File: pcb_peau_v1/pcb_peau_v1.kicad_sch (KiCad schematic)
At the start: 26 parts, among them J1 Conn_01x05, J2 Conn_01x05, J4 Conn_02x08_Top_Bottom, J5 Conn_02x12_Top_Bottom, U2 TLC274, U3 CD74HC4067SM, U4 CD74HC4067SM, U5 CD74HC4067SM, U6 CD74HC4067SM, U7 TLC274, U8 TLC274, U9 TLC274

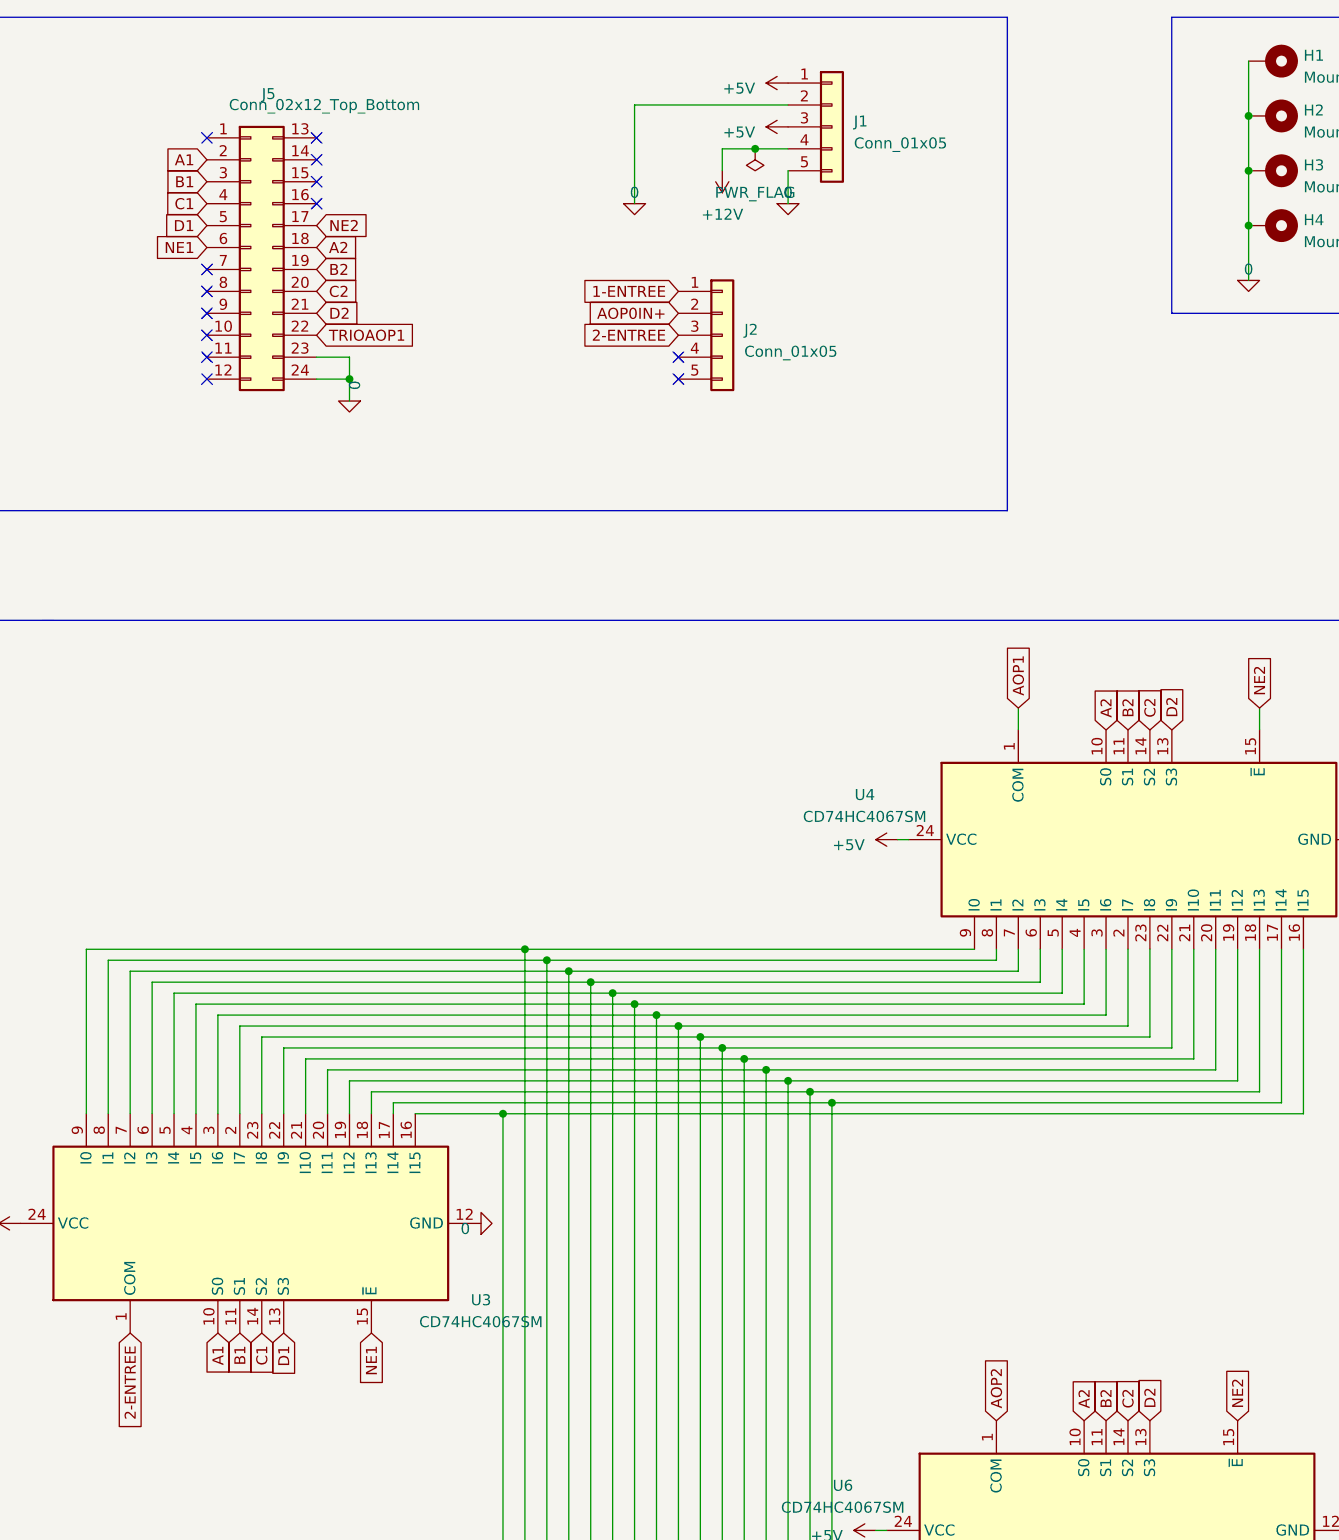
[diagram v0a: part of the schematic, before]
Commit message: PCB corrigé
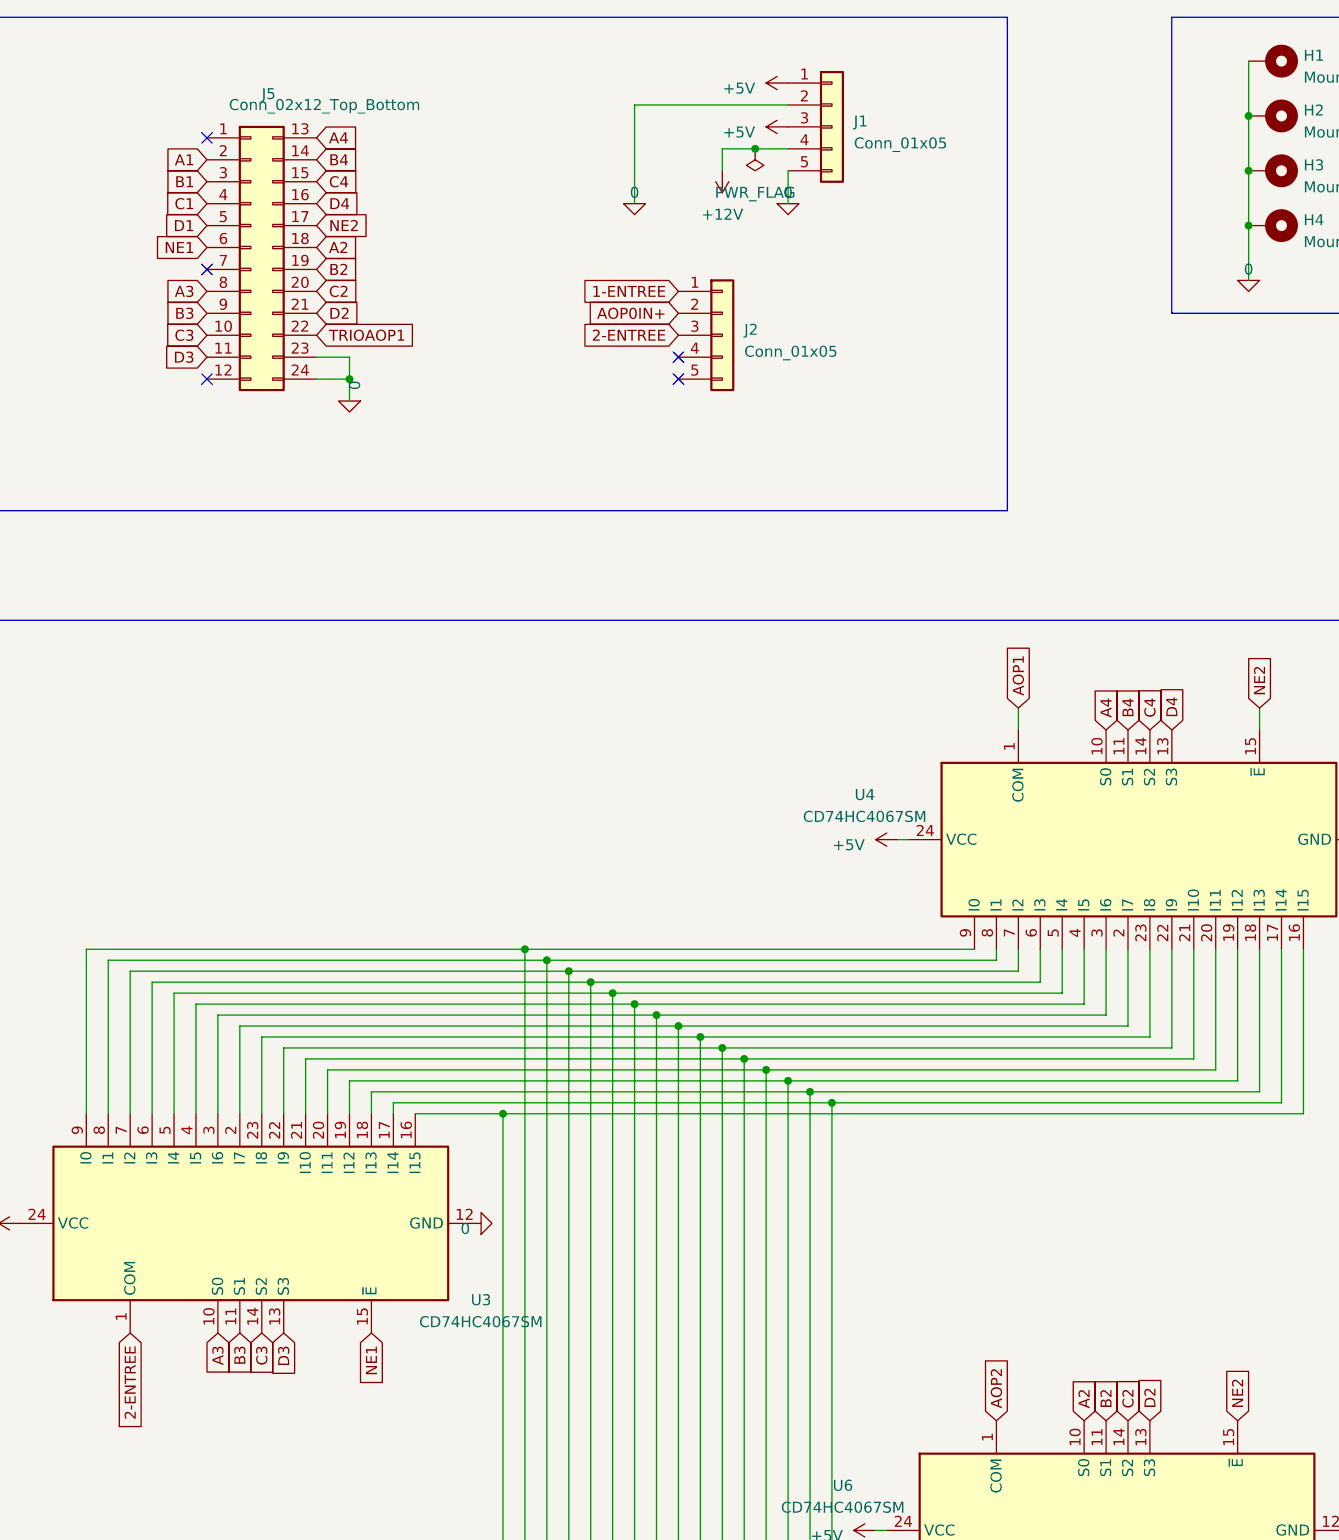
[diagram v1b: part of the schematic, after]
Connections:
- net A1: no longer U3.10 (S0)
- net A2: no longer U4.10 (S0)
- net B1: no longer U3.11 (S1)
- net B2: no longer U4.11 (S1)
- net C1: no longer U3.14 (S2)
- net C2: no longer U4.14 (S2)
- net D1: no longer U3.13 (S3)
- net D2: no longer U4.13 (S3)
- net C3: now reaches J5.10 (Pin_10)
- net C3: now also U3.14 (S2)
- net D3: now reaches J5.11 (Pin_11)
- net D3: now also U3.13 (S3)
- net A4: now reaches J5.13 (Pin_13)
- net A4: now also U4.10 (S0)
- net B4: now reaches J5.14 (Pin_14)
- net B4: now also U4.11 (S1)
- net C4: now reaches J5.15 (Pin_15)
- net C4: now also U4.14 (S2)
- net D4: now reaches J5.16 (Pin_16)
- net D4: now also U4.13 (S3)
- net A3: now reaches J5.8 (Pin_8)
- net A3: now also U3.10 (S0)
- net B3: now reaches J5.9 (Pin_9)
- net B3: now also U3.11 (S1)
- no-connect marks 13 -> 5
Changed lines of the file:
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@@
   (junction (at 96.52 214.63) (diameter 0) (color 0 0 0 0)
   )
-  (no_connect (at 64.77 40.64))
-  (no_connect (at 52.07 60.96))
   (no_connect (at 52.07 35.56))
   (no_connect (at 106.68 63.5))
-  (no_connect (at 52.07 53.34))
-  (no_connect (at 52.07 58.42))
   (no_connect (at 106.68 60.96))
-  (no_connect (at 52.07 55.88))
-  (no_connect (at 64.77 38.1))
-  (no_connect (at 64.77 35.56))
   (no_connect (at 52.07 50.8))
-  (no_connect (at 64.77 43.18))
   (no_connect (at 52.07 63.5))
   (wire (pts (xy 96.52 133.35) (xy 96.52 214.63))
@@
     )
   )
-  (global_label "A1" (shape input) (at 53.34 173.99 270) (fields_autoplaced)
+  (global_label "A3" (shape input) (at 53.34 173.99 270) (fields_autoplaced)
     (effects (font (size 1.27 1.27)) (justify right))
     (property "Intersheetrefs" "${INTERSHEET_REFS}" (at 53.34 179.1939 90)
@@
     )
   )
+  (global_label "C4" (shape input) (at 64.77 40.64 0) (fields_autoplaced)
+    (effects (font (size 1.27 1.27)) (justify left))
+    (property "Intersheetrefs" "${INTERSHEET_REFS}" (at 70.1553 40.64 0)
+      (effects (font (size 1.27 1.27)) (justify left) hide)
+    )
+  )
   (global_label "AOP1" (shape input) (at 232.41 261.62 270) (fields_autoplaced)
     (effects (font (size 1.27 1.27)) (justify right))
@@
     )
   )
-  (global_label "B1" (shape input) (at 55.88 173.99 270) (fields_autoplaced)
+  (global_label "A3" (shape input) (at 52.07 53.34 180) (fields_autoplaced)
+    (effects (font (size 1.27 1.27)) (justify right))
+    (property "Intersheetrefs" "${INTERSHEET_REFS}" (at 46.8661 53.34 0)
+      (effects (font (size 1.27 1.27)) (justify right) hide)
+    )
+  )
+  (global_label "B3" (shape input) (at 55.88 173.99 270) (fields_autoplaced)
     (effects (font (size 1.27 1.27)) (justify right))
     (property "Intersheetrefs" "${INTERSHEET_REFS}" (at 55.88 179.3753 90)
@@
     )
   )
-  (global_label "C1" (shape input) (at 58.42 173.99 270) (fields_autoplaced)
+  (global_label "C3" (shape input) (at 58.42 173.99 270) (fields_autoplaced)
     (effects (font (size 1.27 1.27)) (justify right))
     (property "Intersheetrefs" "${INTERSHEET_REFS}" (at 58.42 179.3753 90)
@@
     )
   )
-  (global_label "D2" (shape input) (at 163.83 104.14 90) (fields_autoplaced)
+  (global_label "D4" (shape input) (at 163.83 104.14 90) (fields_autoplaced)
     (effects (font (size 1.27 1.27)) (justify left))
     (property "Intersheetrefs" "${INTERSHEET_REFS}" (at 163.83 98.7547 90)
@@
     )
   )
-  (global_label "B2" (shape input) (at 158.75 104.14 90) (fields_autoplaced)
+  (global_label "B4" (shape input) (at 158.75 104.14 90) (fields_autoplaced)
     (effects (font (size 1.27 1.27)) (justify left))
     (property "Intersheetrefs" "${INTERSHEET_REFS}" (at 158.75 98.7547 90)
@@
     )
   )
+  (global_label "A4" (shape input) (at 64.77 35.56 0) (fields_autoplaced)
+    (effects (font (size 1.27 1.27)) (justify left))
+    (property "Intersheetrefs" "${INTERSHEET_REFS}" (at 69.9739 35.56 0)
+      (effects (font (size 1.27 1.27)) (justify left) hide)
+    )
+  )
   (global_label "A1" (shape input) (at 52.07 38.1 180) (fields_autoplaced)
     (effects (font (size 1.27 1.27)) (justify right))
@@
     )
   )
+  (global_label "D4" (shape input) (at 64.77 43.18 0) (fields_autoplaced)
+    (effects (font (size 1.27 1.27)) (justify left))
+    (property "Intersheetrefs" "${INTERSHEET_REFS}" (at 70.1553 43.18 0)
+      (effects (font (size 1.27 1.27)) (justify left) hide)
+    )
+  )
   (global_label "D1" (shape input) (at 60.96 254 270) (fields_autoplaced)
     (effects (font (size 1.27 1.27)) (justify right))
@@
     )
   )
+  (global_label "B3" (shape input) (at 52.07 55.88 180) (fields_autoplaced)
+    (effects (font (size 1.27 1.27)) (justify right))
+    (property "Intersheetrefs" "${INTERSHEET_REFS}" (at 46.6847 55.88 0)
+      (effects (font (size 1.27 1.27)) (justify right) hide)
+    )
+  )
   (global_label "A2" (shape input) (at 153.67 184.15 90) (fields_autoplaced)
     (effects (font (size 1.27 1.27)) (justify left))
@@
     )
   )
+  (global_label "B4" (shape input) (at 64.77 38.1 0) (fields_autoplaced)
+    (effects (font (size 1.27 1.27)) (justify left))
+    (property "Intersheetrefs" "${INTERSHEET_REFS}" (at 70.1553 38.1 0)
+      (effects (font (size 1.27 1.27)) (justify left) hide)
+    )
+  )
   (global_label "B1" (shape input) (at 52.07 40.64 180) (fields_autoplaced)
     (effects (font (size 1.27 1.27)) (justify right))
@@
     )
   )
+  (global_label "D3" (shape input) (at 52.07 60.96 180) (fields_autoplaced)
+    (effects (font (size 1.27 1.27)) (justify right))
+    (property "Intersheetrefs" "${INTERSHEET_REFS}" (at 46.6847 60.96 0)
+      (effects (font (size 1.27 1.27)) (justify right) hide)
+    )
+  )
   (global_label "TRIOAOP1" (shape input) (at 64.77 58.42 0) (fields_autoplaced)
     (effects (font (size 1.27 1.27)) (justify left))
@@
     )
   )
-  (global_label "D1" (shape input) (at 60.96 173.99 270) (fields_autoplaced)
+  (global_label "C3" (shape input) (at 52.07 58.42 180) (fields_autoplaced)
+    (effects (font (size 1.27 1.27)) (justify right))
+    (property "Intersheetrefs" "${INTERSHEET_REFS}" (at 46.6847 58.42 0)
+      (effects (font (size 1.27 1.27)) (justify right) hide)
+    )
+  )
+  (global_label "D3" (shape input) (at 60.96 173.99 270) (fields_autoplaced)
     (effects (font (size 1.27 1.27)) (justify right))
     (property "Intersheetrefs" "${INTERSHEET_REFS}" (at 60.96 179.3753 90)
@@
     )
   )
-  (global_label "C2" (shape input) (at 161.29 104.14 90) (fields_autoplaced)
+  (global_label "C4" (shape input) (at 161.29 104.14 90) (fields_autoplaced)
     (effects (font (size 1.27 1.27)) (justify left))
     (property "Intersheetrefs" "${INTERSHEET_REFS}" (at 161.29 98.7547 90)
@@
     )
   )
-  (global_label "A2" (shape input) (at 156.21 104.14 90) (fields_autoplaced)
+  (global_label "A4" (shape input) (at 156.21 104.14 90) (fields_autoplaced)
     (effects (font (size 1.27 1.27)) (justify left))
     (property "Intersheetrefs" "${INTERSHEET_REFS}" (at 156.21 98.9361 90)
